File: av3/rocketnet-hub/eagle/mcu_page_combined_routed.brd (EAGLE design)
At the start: 112.7 x 76.3 mm, 446 parts, among them J1 ROCKETNET-CONNECTOR-16M, J10 UART Header, J11 I2C Header, J12 BOOT1 Jumper, J13 PGOOD Jumper, J14 ROCKETNET-UMBILICAL-18, J15 Auxiliary Header, J16 Auxiliary Header, J17 Auxiliary Header, J18 Auxiliary Header, J19 Auxiliary Header, J2 ROCKETNET-CONNECTOR-16M, J20 Auxiliary Header, J21 Auxiliary Header, J22 Debug Header, J3 ROCKETNET-CONNECTOR-16M, J4 ROCKETNET-CONNECTOR-16M, J5 BOOT0 Jumper, J6 ROCKETNET-CONNECTOR-16M, J7 ROCKETNET-CONNECTOR-16M, J8 ROCKETNET-CONNECTOR-16M, J9 ROCKETNET-BATTERY-14, Q2 FDS6680ASOIC8, Q3 FDS6680ASOIC8, Q4 FDS6680ASOIC8, Q5 SIS412DNSOP-8, Q6 BSS138W-7-F, Q7 SIS412DNSOP-8, T1 BSS84, T10 ALT4532, T11 ALT4532, T12 ALT4532, T13 ALT4532, T14 ALT4532, T15 ALT4532, T16 ALT4532, T17 ALT4532, T18 ALT4532, T19 BSS84, T2 NDS335N, T20 NDS335N, T3 ALT4532, T4 ALT4532, T5 ALT4532, T6 ALT4532, T7 ALT4532, T8 ALT4532, T9 ALT4532, U1 STM32F407V100-PIN_QFP, U10 TPS2420QFN-16, U11 TPS2420QFN-16, U12 TPS2420QFN-16, U13 TPS2420QFN-16, U14 MAX4734ETC+, U15 MAX4734ETC+, U2 BQ24725QFN-20, U3 SN65220DBV, U4 KS8999, U5 LTM8023, U6 MIC37101-2.1YM, U7 TPS2420QFN-16, U8 TPS2420QFN-16, U9 TPS2420QFN-16

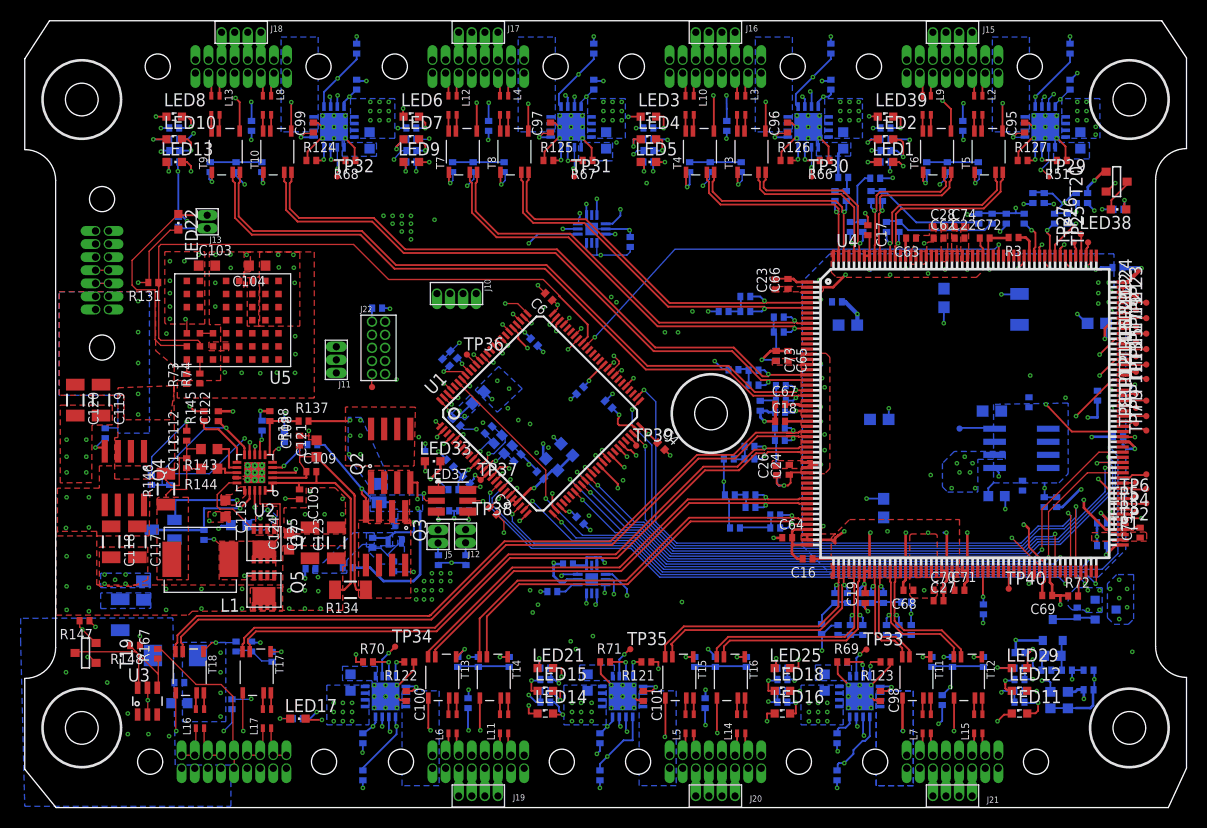
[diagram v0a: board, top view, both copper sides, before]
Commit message: Fixed routes
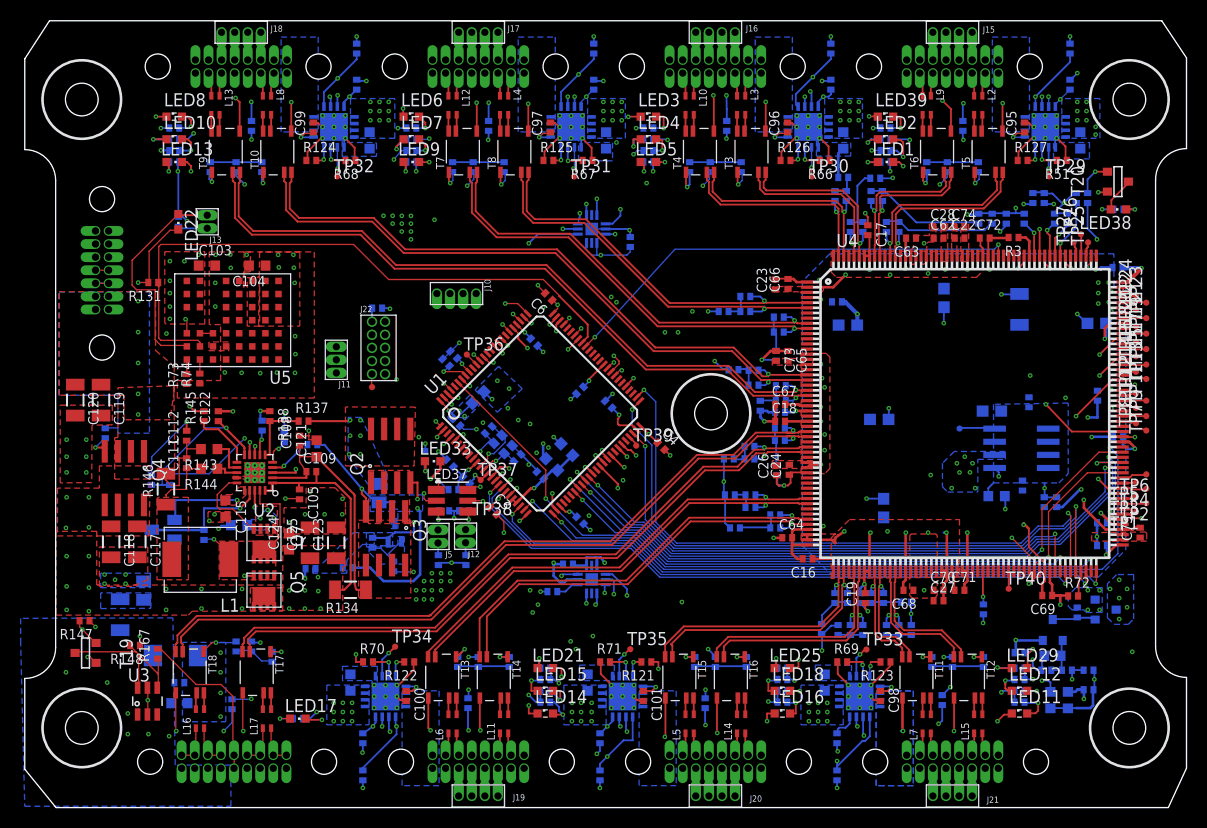
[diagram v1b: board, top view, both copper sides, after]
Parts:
- moved T20 0.13 mm to (106.0, 60.6)
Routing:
- net NODE4_IMON_IN: track 42.2 -> 40.1 mm
- net N$14: track 4.81 -> 3.61 mm
- net NODE1_LTCH: track 3.58 -> 2.85 mm
- net +2V1: track 167.9 -> 168.5 mm
- net N$19: track 5.75 -> 5.76 mm, vias 2 -> 1

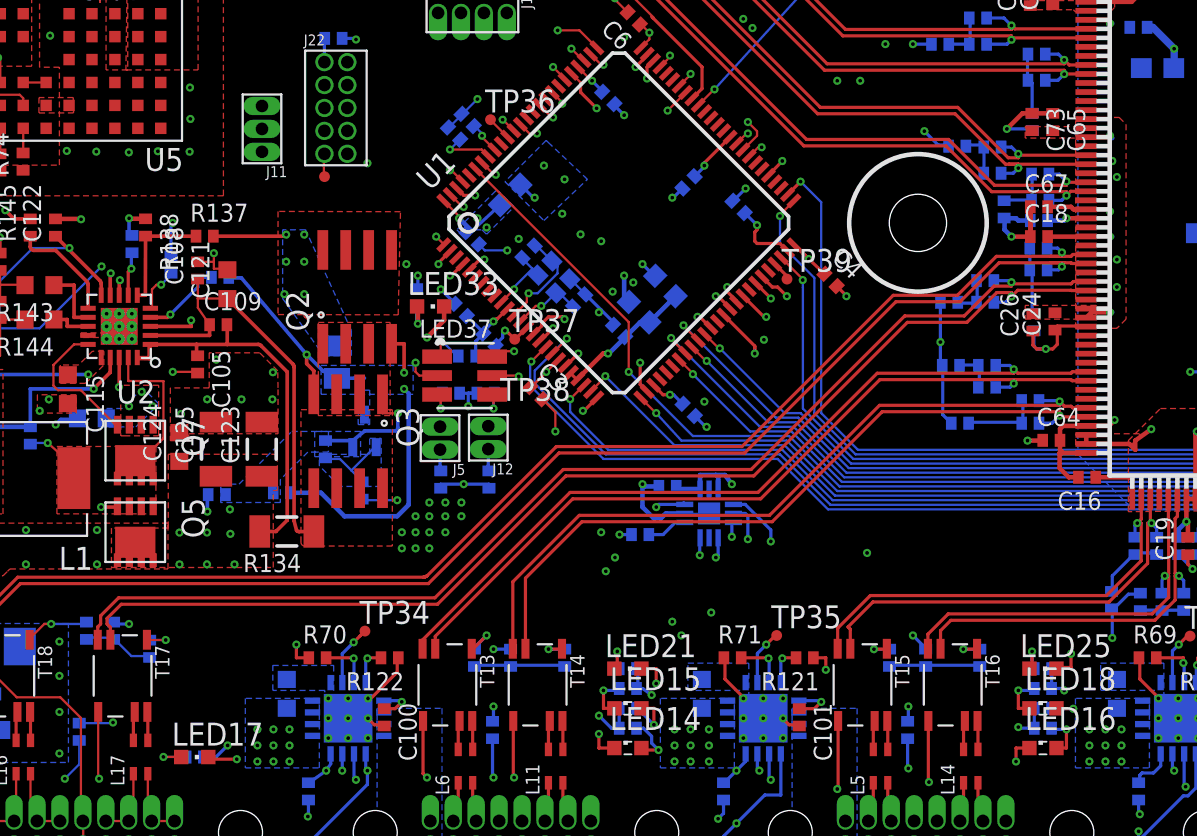
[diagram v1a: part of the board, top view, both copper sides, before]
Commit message: Fixed more routes
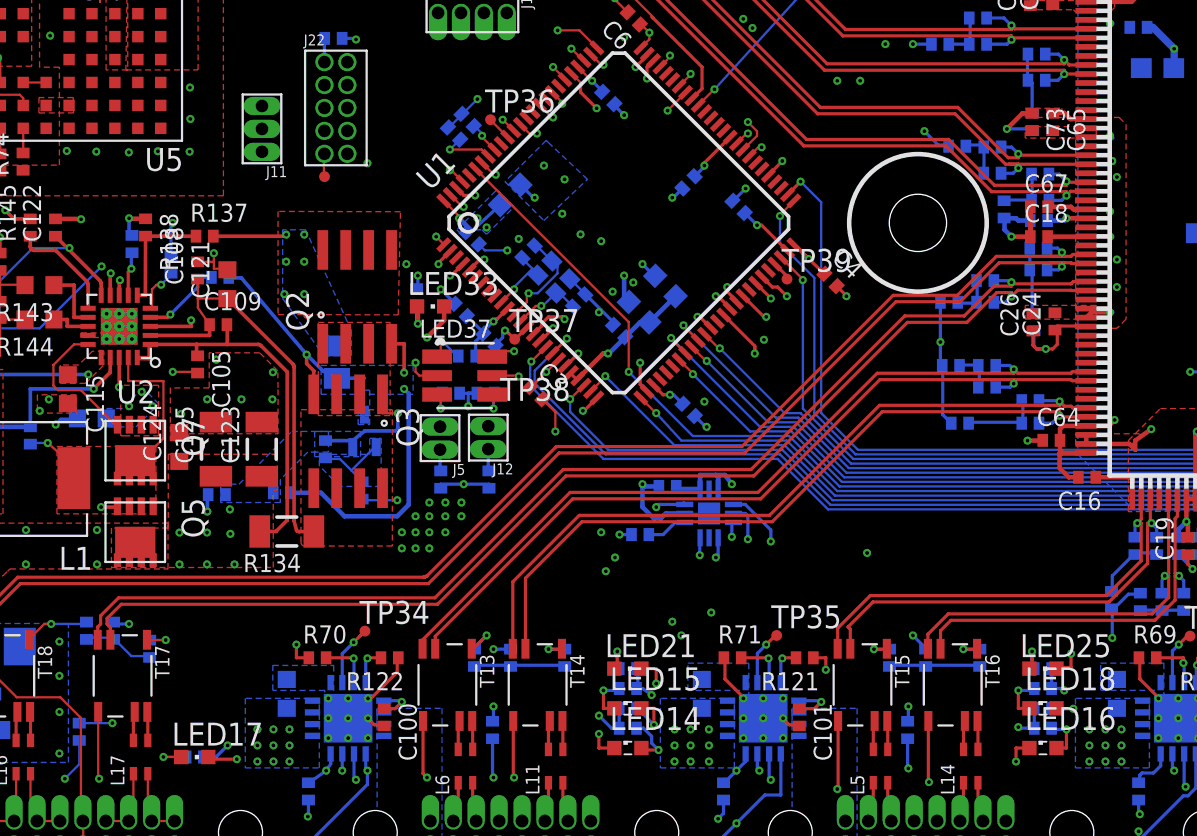
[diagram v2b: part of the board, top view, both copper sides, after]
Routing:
- net GND: track 258.7 -> 259.6 mm
- net N$12: track 3.95 -> 3.25 mm
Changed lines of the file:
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@@
 <layer number="49" name="Reference" color="7" fill="1" visible="no" active="yes"/>
 <layer number="50" name="dxf" color="7" fill="1" visible="no" active="no"/>
-<layer number="51" name="tDocu" color="7" fill="1" visible="no" active="yes"/>
-<layer number="52" name="bDocu" color="7" fill="1" visible="no" active="yes"/>
+<layer number="51" name="tDocu" color="7" fill="1" visible="yes" active="yes"/>
+<layer number="52" name="bDocu" color="7" fill="1" visible="yes" active="yes"/>
 <layer number="53" name="tGND_GNDA" color="7" fill="1" visible="no" active="no"/>
 <layer number="54" name="bGND_GNDA" color="7" fill="1" visible="no" active="no"/>
@@
 <attribute name="VALUE" x="59.064" y="34.604" size="0.0254" layer="27"/>
 </element>
-<element name="J11" library="headers" package="1.27MM_3X1" value="I2C Header" x="30.226" y="42.672" rot="R180"/>
-<element name="R18" library="rcl_custom" package="0402-B-NOSILK" value="10k" x="51.181" y="20.828" rot="MR180"/>
+<element name="J11" library="headers" package="1.27MM_3X1" value="I2C Header" x="30.226" y="42.672" smashed="yes" rot="R180">
+<attribute name="NAME" x="31.626" y="41.242" size="0.6096" layer="25" rot="R180"/>
+<attribute name="VALUE" x="31.626" y="45.972" size="0.6096" layer="27" rot="R180"/>
+</element>
+<element name="R18" library="rcl_custom" package="0402-B-NOSILK" value="10k" x="51.181" y="20.828" smashed="yes" rot="MR180">
+<attribute name="NAME" x="50.381" y="20.028" size="1" layer="26" ratio="10" rot="MR180"/>
+<attribute name="VALUE" x="50.381" y="22.678" size="1" layer="28" ratio="10" rot="MR180"/>
+</element>
 </elements>
 <signals>
@@
 <contactref element="U1" pad="49"/>
 <wire x1="57.658" y1="37.973" x2="57.023" y2="38.608" width="0.1778" layer="16"/>
-<wire x1="57.658" y1="37.719" x2="57.658" y2="37.973" width="0.1778" layer="1"/>
-<wire x1="57.531" y1="37.592" x2="57.658" y2="37.719" width="0.1778" layer="1"/>
-<wire x1="57.531" y1="37.084" x2="57.531" y2="37.592" width="0.1778" layer="1"/>
-<wire x1="57.658" y1="36.957" x2="57.531" y2="37.084" width="0.1778" layer="1"/>
-<wire x1="58.928" y1="36.957" x2="57.658" y2="36.957" width="0.1778" layer="1"/>
-<wire x1="59.309" y1="36.576" x2="58.928" y2="36.957" width="0.1778" layer="1"/>
 <wire x1="57.023" y1="38.608" x2="56.9764125" y2="38.6435875" width="0.1778" layer="16"/>
 <wire x1="59.309" y1="36.576" x2="59.34795" y2="36.530221875" width="0.1778" layer="1"/>
 <via x="57.658" y="37.973" extent="1-16" drill="0.2032" diameter="0.4572"/>
+<wire x1="59.309" y1="36.576" x2="57.912" y2="37.973" width="0.1778" layer="1"/>
+<wire x1="57.912" y1="37.973" x2="57.658" y2="37.973" width="0.1778" layer="1"/>
 </signal>
 <signal name="GND" class="1">
@@
 <wire x1="107.696" y1="40.894" x2="106.172" y2="39.37" width="0.127" layer="16"/>
 <via x="11.176" y="16.51" extent="1-16" drill="0.2032" diameter="0.4572"/>
-<via x="21.971" y="10.414" extent="1-16" drill="0.2032" diameter="0.4572"/>
 <via x="25.281" y="29.845" extent="1-16" drill="0.2032" diameter="0.4572"/>
 <via x="37.719" y="22.733" extent="1-16" drill="0.2032" diameter="0.4572"/>
@@
 <via x="23.56" y="28.74" extent="1-16" drill="0.2032" diameter="0.4572"/>
 <wire x1="20.1" y1="10.38" x2="21.937" y2="10.38" width="0.127" layer="16"/>
-<wire x1="21.937" y1="10.38" x2="21.971" y2="10.414" width="0.127" layer="16"/>
 <wire x1="92.71" y1="54.356" x2="92.71" y2="55.118" width="0.1778" layer="1"/>
 <wire x1="92.964" y1="54.102" x2="92.71" y2="54.356" width="0.1778" layer="1"/>
@@
 <wire x1="71.374" y1="38.354" x2="71.374" y2="37.719" width="0.254" layer="16"/>
 <wire x1="71.374" y1="37.719" x2="71.755" y2="37.338" width="0.254" layer="16"/>
-<wire x1="74.041" y1="44.168" x2="72.898" y2="44.168" width="0.254" layer="1"/>
 <wire x1="72.362" y1="44.168" x2="71.501" y2="43.307" width="0.254" layer="1"/>
 <wire x1="92.546" y1="57.48" x2="92.47" y2="57.404" width="0.254" layer="16"/>
@@
 <via x="104.14" y="59.563" extent="1-16" drill="0.2032" diameter="0.4572"/>
 <wire x1="104.14" y1="59.563" x2="104.013" y2="59.563" width="0.1778" layer="2"/>
+<via x="21.937" y="10.38" extent="1-16" drill="0.2032" diameter="0.4572"/>
+<wire x1="21.937" y1="10.38" x2="21.971" y2="10.38" width="0.127" layer="2"/>
+<wire x1="21.971" y1="10.38" x2="21.971" y2="10.414" width="0.127" layer="2"/>
+<wire x1="74.041" y1="44.168" x2="74.069" y2="44.196" width="0.1778" layer="1"/>
+<wire x1="74.069" y1="44.196" x2="74.676" y2="44.196" width="0.254" layer="1"/>
+<wire x1="74.676" y1="44.196" x2="75.022" y2="43.85" width="0.254" layer="1"/>
+<wire x1="75.022" y1="43.85" x2="75.9" y2="43.85" width="0.254" layer="1"/>
+<polygon width="0.1778" layer="1">
+<vertex x="72.517" y="44.45"/>
+<vertex x="74.549" y="44.45"/>
+<vertex x="74.549" y="43.942"/>
+<vertex x="72.517" y="43.942"/>
+</polygon>
 </signal>
 <signal name="+3V3" class="1">
